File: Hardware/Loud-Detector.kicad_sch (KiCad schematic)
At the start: 27 parts, among them J1 TP4056, J2 ON_OFF, J3 VIN+, J4 VIN-, J5 VOUT+, J6 VOUT-, J7 KY-037, J8 BUZZER, Q1 BC557, Q2 BC547, U1 ATtiny85, U2 MT3608_Module

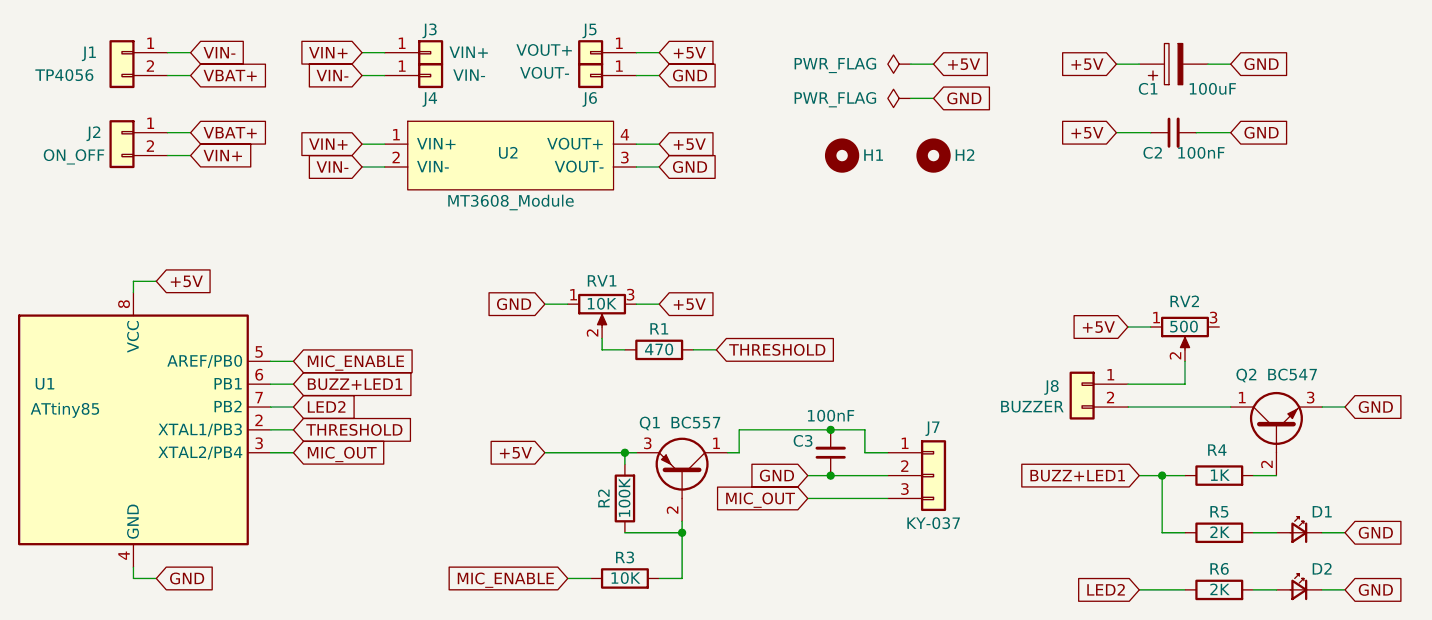
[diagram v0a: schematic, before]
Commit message: PCB minor improvements
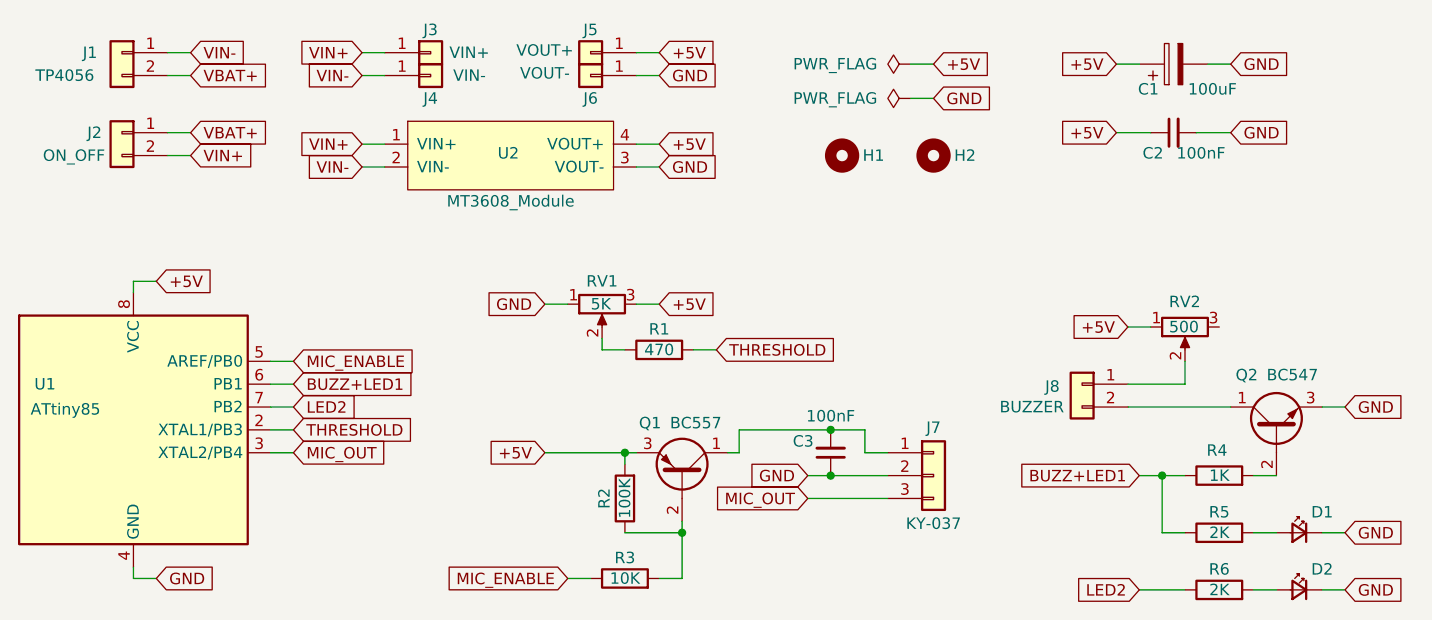
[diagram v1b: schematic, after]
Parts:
- RV1: value 10K -> 5K
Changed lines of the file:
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@@
 	(wire
 		(pts
+			(xy 132.08 90.17) (xy 134.62 90.17)
+		)
+		(stroke
+			(width 0)
+			(type default)
+		)
+	)
+	(wire
+		(pts
 			(xy 210.82 115.57) (xy 213.36 115.57)
 		)
@@
 	(wire
 		(pts
-			(xy 132.08 90.17) (xy 134.62 90.17)
-		)
-		(stroke
-			(width 0)
-			(type default)
-		)
-	)
-	(wire
-		(pts
 			(xy 147.32 115.57) (xy 147.32 114.3)
 		)
@@
 			)
 		)
-		(property "Value" "10K"
-			(at 136.652 90.17 90)
+		(property "Value" "5K"
+			(at 137.16 90.17 90)
 			(effects
 				(font

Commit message: PCB minor improvements
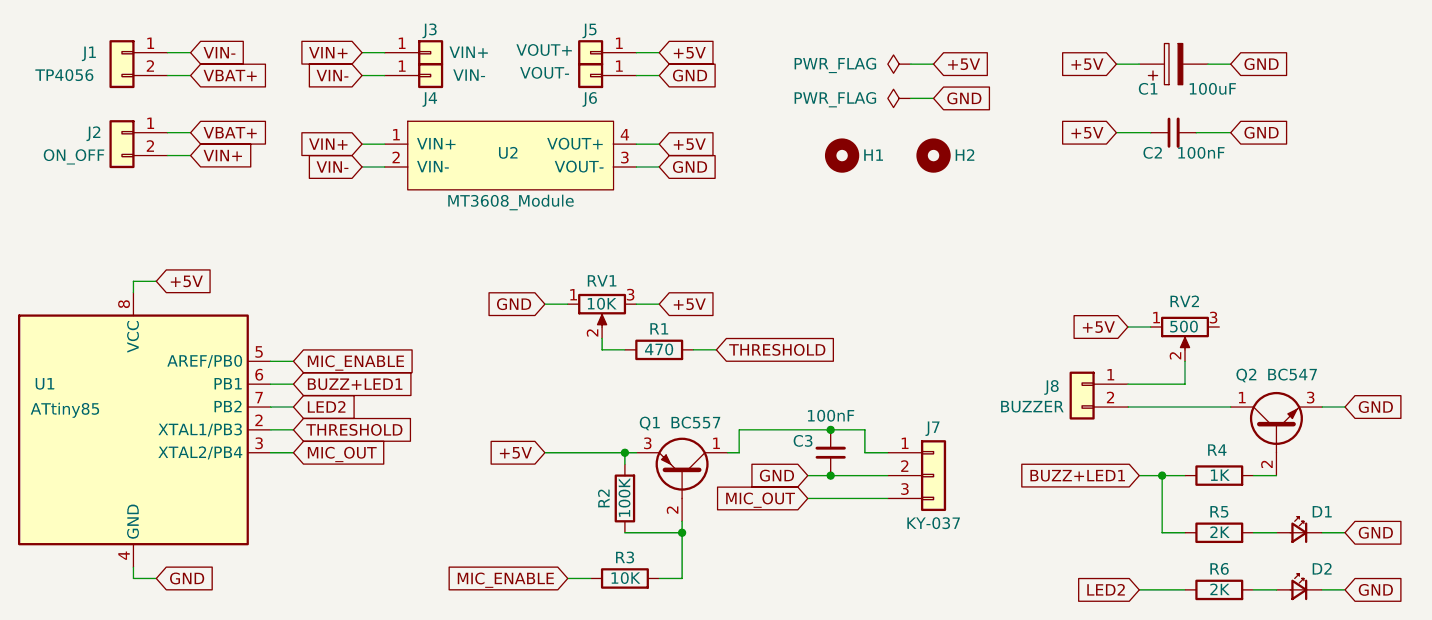
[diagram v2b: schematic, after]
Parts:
- RV1: value 5K -> 10K
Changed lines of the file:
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@@
+		)
+	)
+	(global_label "MIC_OUT"
+		(shape input)
+		(at 161.29 111.76 180)
+		(fields_autoplaced yes)
+		(effects
+			(font
+				(size 1.27 1.27)
+			)
+			(justify right)
+		)
+		(property "Intersheetrefs" "${INTERSHEET_REFS}"
+			(at 150.3824 111.76 0)
+			(effects
+				(font
+					(size 1.27 1.27)
+				)
+				(justify right)
+				(hide yes)
+			)
+		)
+	)
+	(global_label "VBAT+"
+		(shape input)
+		(at 92.71 64.77 0)
+		(fields_autoplaced yes)
+		(effects
+			(font
+				(size 1.27 1.27)
+			)
+			(justify left)
+		)
+		(property "Intersheetrefs" "${INTERSHEET_REFS}"
+			(at 101.6824 64.77 0)
+			(effects
+				(font
+					(size 1.27 1.27)
+				)
+				(justify left)
+				(hide yes)
+			)
+		)
+	)
+	(global_label "GND"
+		(shape input)
+		(at 132.08 90.17 180)
+		(fields_autoplaced yes)
+		(effects
+			(font
+				(size 1.27 1.27)
+			)
+			(justify right)
+		)
+		(property "Intersheetrefs" "${INTERSHEET_REFS}"
+			(at 125.2243 90.17 0)
+			(effects
+				(font
+					(size 1.27 1.27)
+				)
+				(justify right)
+				(hide yes)
+			)
 		)
 	)
@@
 				)
 				(justify left)
-				(hide yes)
-			)
-		)
-	)
-	(global_label "MIC_OUT"
-		(shape input)
-		(at 161.29 111.76 180)
-		(fields_autoplaced yes)
-		(effects
-			(font
-				(size 1.27 1.27)
-			)
-			(justify right)
-		)
-		(property "Intersheetrefs" "${INTERSHEET_REFS}"
-			(at 150.3824 111.76 0)
-			(effects
-				(font
-					(size 1.27 1.27)
-				)
-				(justify right)
-				(hide yes)
-			)
-		)
-	)
-	(global_label "VBAT+"
-		(shape input)
-		(at 92.71 64.77 0)
-		(fields_autoplaced yes)
-		(effects
-			(font
-				(size 1.27 1.27)
-			)
-			(justify left)
-		)
-		(property "Intersheetrefs" "${INTERSHEET_REFS}"
-			(at 101.6824 64.77 0)
-			(effects
-				(font
-					(size 1.27 1.27)
-				)
-				(justify left)
-				(hide yes)
-			)
-		)
-	)
-	(global_label "GND"
-		(shape input)
-		(at 132.08 90.17 180)
-		(fields_autoplaced yes)
-		(effects
-			(font
-				(size 1.27 1.27)
-			)
-			(justify right)
-		)
-		(property "Intersheetrefs" "${INTERSHEET_REFS}"
-			(at 125.2243 90.17 0)
-			(effects
-				(font
-					(size 1.27 1.27)
-				)
-				(justify right)
 				(hide yes)
 			)
@@
 			)
 		)
-		(property "Value" "5K"
-			(at 137.16 90.17 90)
-			(effects
-				(font
+		(property "Value" "10K"
+			(at 136.652 90.17 90)
+			(effects
+				(font
